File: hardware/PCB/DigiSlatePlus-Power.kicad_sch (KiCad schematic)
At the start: 29 parts, among them Q2 FS8205A, U11 KA78M05_TO252, U12 LM2596S-ADJ, U13 LD1117S33TR_SOT223, U14 TP4056, U15 DW01A

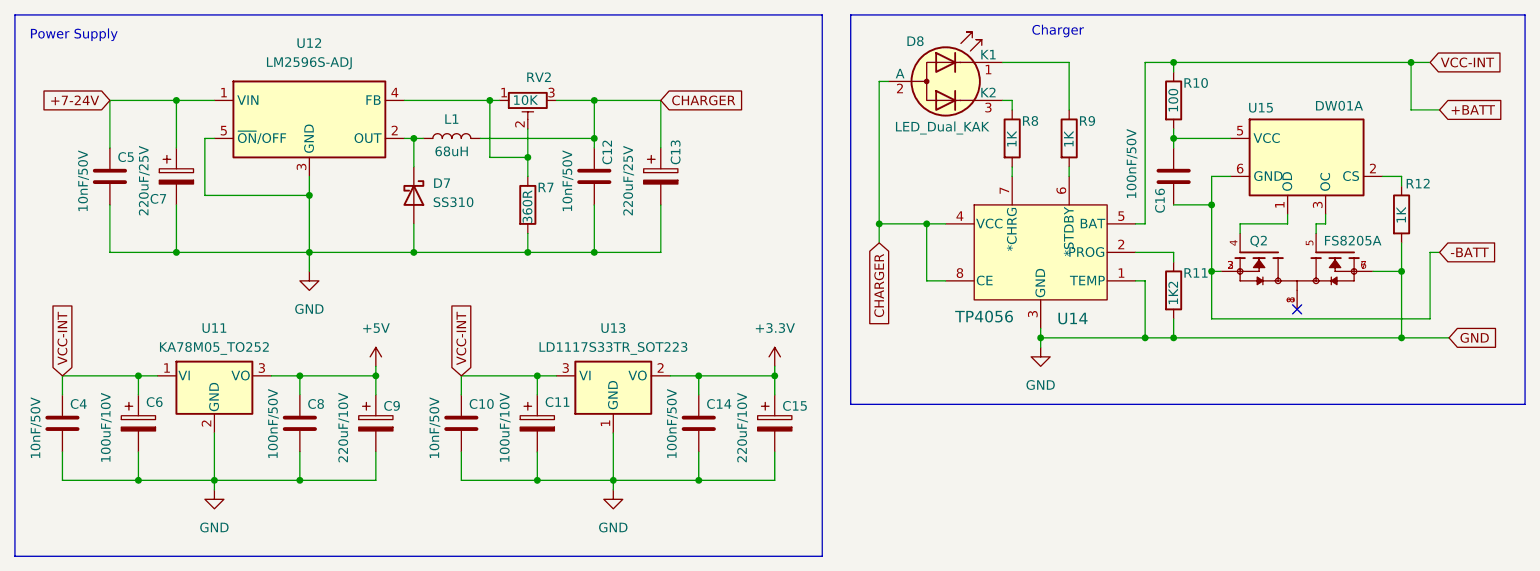
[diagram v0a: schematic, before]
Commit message: change page structure
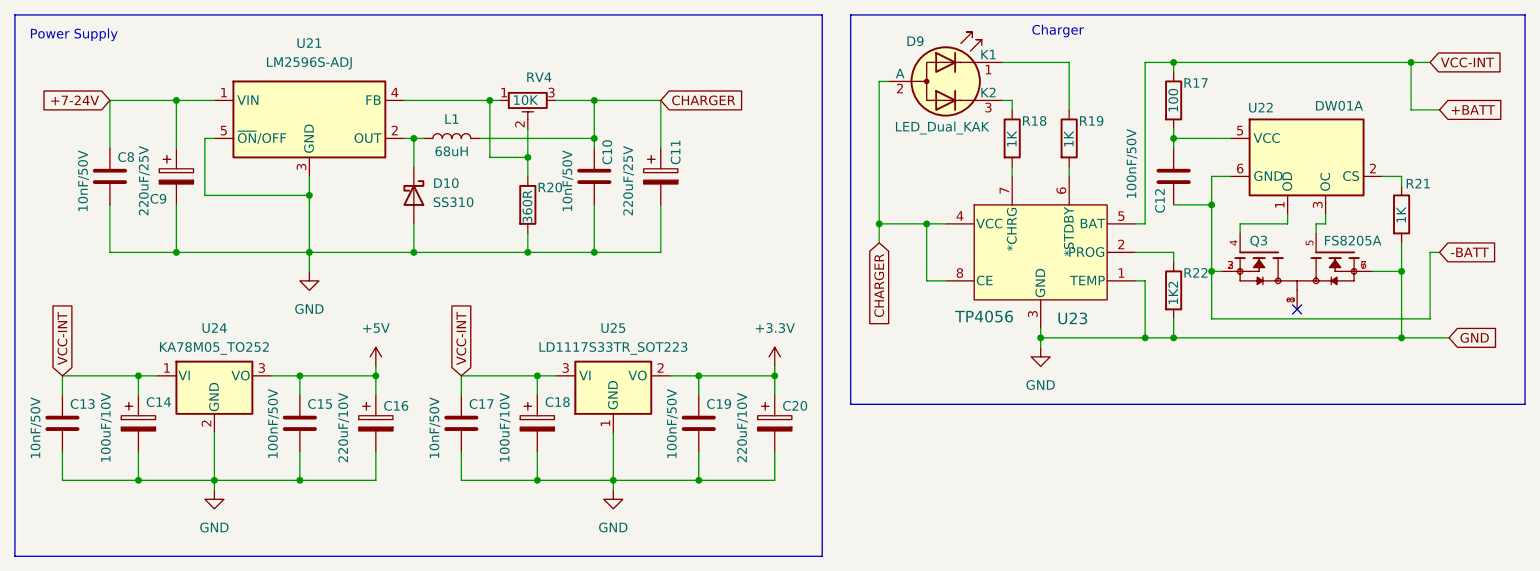
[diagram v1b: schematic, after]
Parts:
- renumbered C12 to C10, C13 to C11, C16 to C12, C4 to C13, C6 to C14, C8 to C15, C9 to C16, C10 to C17, C11 to C18, C14 to C19, C15 to C20, C5 to C8, C7 to C9, D7 to D10, D8 to D9, Q2 to Q3, R10 to R17, R8 to R18, R9 to R19, R7 to R20, R12 to R21, R11 to R22, RV2 to RV4, U12 to U21, U15 to U22, U14 to U23, U11 to U24, U13 to U25
